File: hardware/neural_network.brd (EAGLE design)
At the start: 31.2 x 39 mm, 32 parts, among them IC1 74AHC1G04DBV, IC2 74AHC1G04DBV, IC3 74AHCT1G14DBV, IC4 74AHCT1G14DBV

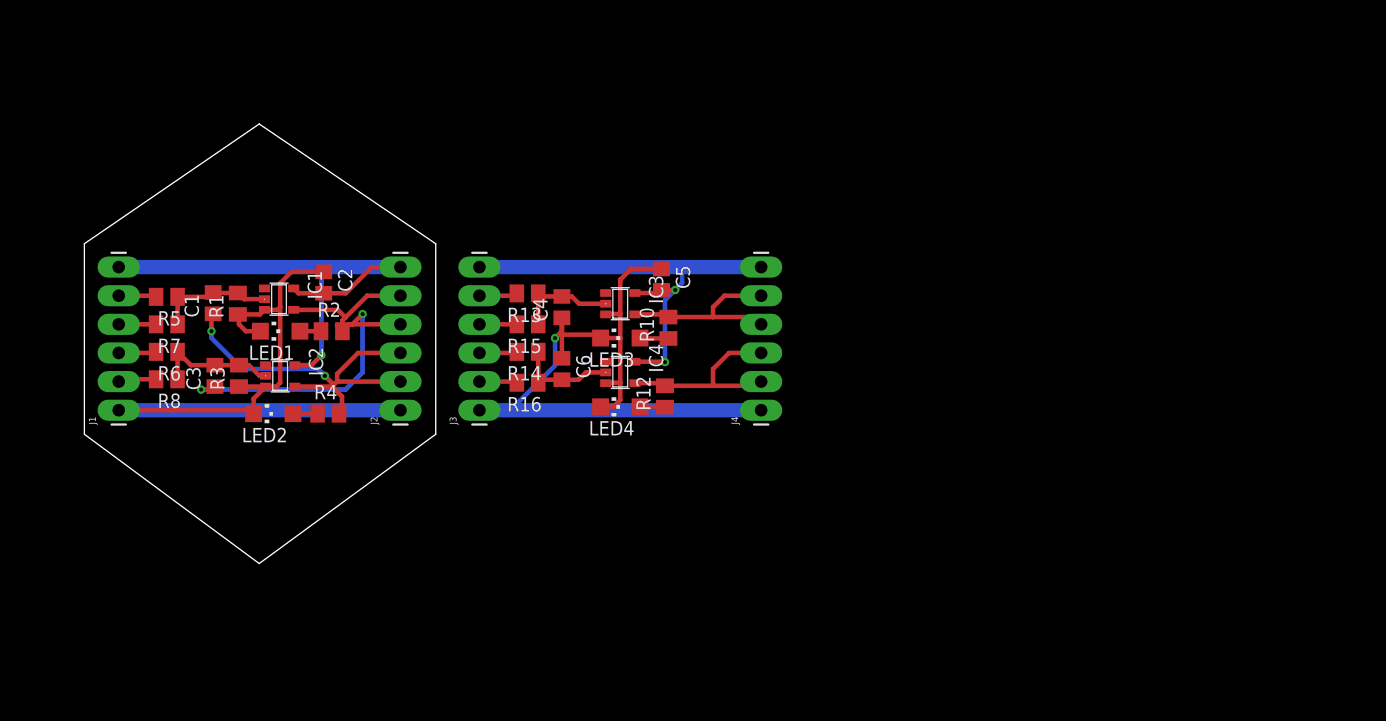
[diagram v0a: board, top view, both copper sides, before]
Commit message: hw
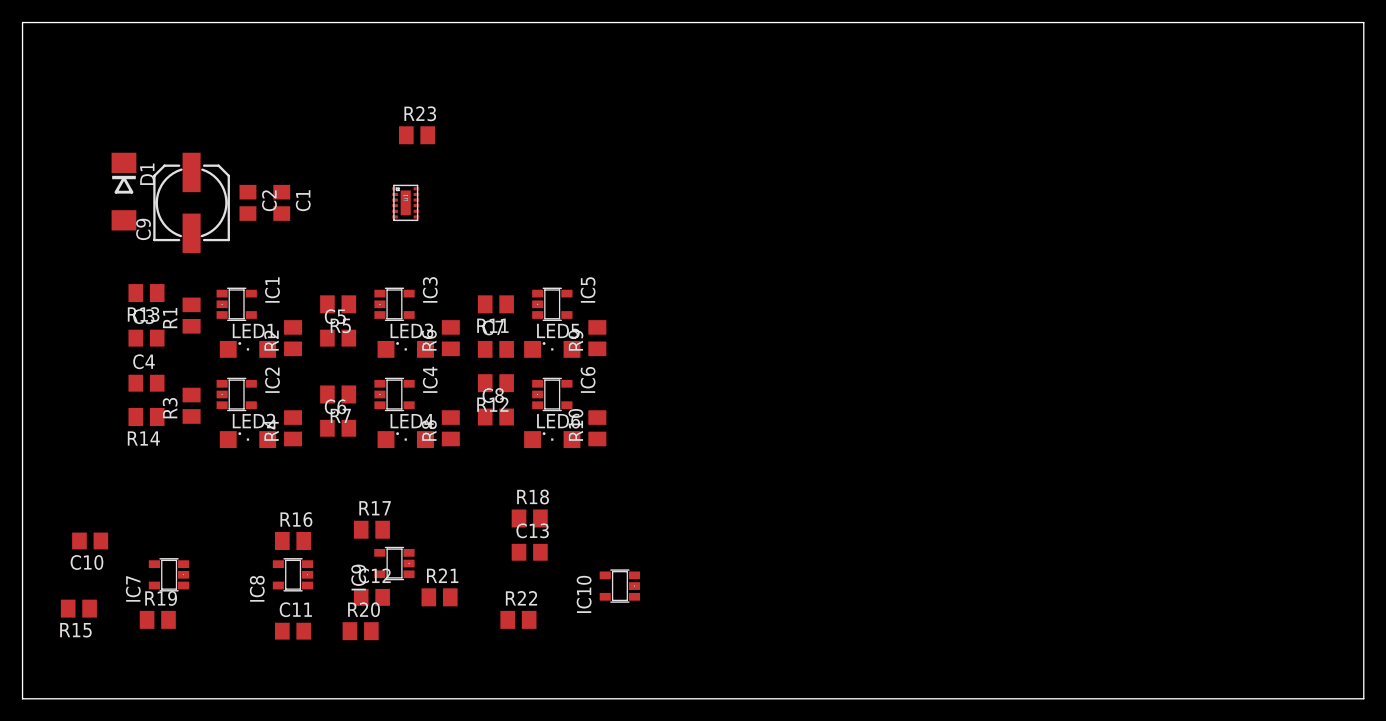
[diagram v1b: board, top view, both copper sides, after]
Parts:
- removed J1, J2, J3, J4: (no value), SparkFun-Connectors:1X06_LONGPADS
- added C10, C11, C12, C13, C7, C8: 100n, resistor:C0805
- added C9: 22uF, resistor:153CLV-0605
- added D1: (no value), diode:DO214AA
- added IC10, IC5, IC6, IC7, IC8, IC9: 74AHC1G14DBV, 74xx-little-de:SOT23-5
- added LED5, LED6: (no value), led:SML1206
- added R11, R17, R18, R19, R20, R21, R22: 1M, resistor:M0805
- added R23, R9: 4k7, resistor:M0805
- added U1: DRV8836, balto:12WSON
- C2: value 100n -> 10uF
- IC1, IC2: value 74AHC1G04DBV -> 74AHC1G14DBV
- IC3, IC4: value 74AHCT1G14DBV -> 74AHC1G14DBV
- LED1, LED2, LED3, LED4: device led:CHIPLED_1206 -> led:SML1206
- R12: value 4k7 -> 1M
- R6, R8: value 1M -> 4k7
- moved R15 47.1 mm to (5.00, 8.00)
- moved C4 37.5 mm to (11.0, 28.0), turned to 0 degrees
- moved R14 34.3 mm to (11.0, 25.0)
- moved R13 33.8 mm to (11.0, 36.0)
- moved C5 29.2 mm to (28.0, 32.0), turned to 0 degrees
- moved R8 25.6 mm to (38.0, 24.0), turned to 90 degrees
- moved R6 25.2 mm to (38.0, 32.0), turned to 90 degrees
- moved R16 25.1 mm to (24.0, 14.0), turned to 0 degrees
- moved C6 20.5 mm to (28.0, 24.0), turned to 0 degrees
- moved IC4 20.1 mm to (33.0, 27.0)
- moved IC3 20.0 mm to (33.0, 35.0)
- moved LED4 19.3 mm to (34.0, 23.0), turned to 0 degrees
- moved LED3 19.1 mm to (34.0, 31.0), turned to 0 degrees
- moved R7 16.4 mm to (28.0, 27.0)
- moved R5 15.2 mm to (28.0, 35.0)
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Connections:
- removed net +3V3: C2.2, C5.2, IC1.5, IC2.5, IC3.5, IC4.5, J1.6, J2.6, J3.6, J4.6
- removed net IN0: J1.5, R5.2
- removed net IN0_: J3.5, R13.2
- removed net IN1: J1.4, R7.2
- removed net IN1_: J3.4, R15.2
- removed net IN2: J1.3, R6.2
- removed net IN2_: J3.3, R14.2
- removed net IN3: J1.2, R8.2
- removed net IN3_: J3.2, R16.2
- removed net N$7 (its old number): LED4.A, R12.1
- removed net OUT0: C3.1, IC1.4, J2.4, J2.5, R2.2
- removed net OUT0_: IC3.4, J4.4, J4.5, R10.2
- removed net OUT1: C1.1, IC2.4, J2.2, J2.3, R4.2
- removed net OUT1_: IC4.4, J4.2, J4.3, R12.2
- new net B_OUT_0: C4.1, IC1.4, R2.2, R5.2, U1.10
- new net B_OUT_1: C3.1, IC2.4, R4.2, R7.2, U1.9
- new net IN_0: R13.2
- new net IN_1: R14.2
- new net N$10: C7.2, IC5.2, R11.1
- new net N$11: LED5.A, R9.1
- new net N$12: C8.2, IC6.2, R12.1
- new net N$13: LED6.A, R10.1
- new net N$14: C10.2, IC7.2, R15.2, R19.1
- new net N$15: C10.1
- new net N$16: IC7.4
- new net N$17: C11.2, IC8.2, R16.2, R20.1
- new net N$18: C11.1
- new net N$19: IC8.4
- new net N$20: C12.2, IC9.2, R17.2, R21.1
- new net N$21: C12.1
- new net N$22: IC9.4
- new net N$23: C13.2, IC10.2, R18.2, R22.1
- new net N$24: C13.1
- new net N$25: IC10.4
- new net N$26: R19.2
- new net N$27: R20.2
- new net N$28: R21.2
- new net N$29: R22.2
- new net N$32: R23.2, U1.12
- new net N$33: U1.3
- new net N$36: U1.2
- new net N$37: U1.4
- new net N$38: U1.5
- new net N$8: C6.2, IC4.2, R7.1
- new net N$9: LED4.A, R8.1
- new net S0_OUT_0: IC3.4, R11.2, R6.2, U1.8
- new net S0_OUT_1: IC4.4, R12.2, R8.2, U1.7
- new net S1_OUT_0: IC5.4, R9.2
- new net S1_OUT_1: IC6.4, R10.2
- new net VCC: D1.A, IC10.5, IC7.5, IC8.5, IC9.5, U1.1
- net GND: now also C1.2, C2.2, C7.1, C8.1, C9.-, IC10.3, IC5.3, IC6.3, IC7.3, IC8.3, IC9.3, LED5.C, LED6.C, R15.1, R16.1, R17.1, R18.1, U1.11, U1.TH; no longer C2.1, C4.1, J1.1, J2.1, J3.1, J4.1
- net N$1: now also C1.1, C2.1, C9.+, D1.C, IC1.5, IC2.5, IC3.5, IC4.5, IC5.5, IC6.5; no longer C1.2, IC1.2, R1.2, R5.1, R7.1
- net N$2: now also C3.2, IC1.2, R1.2; no longer C4.2, IC3.2, R15.1
- net N$3: now also C5.2, IC3.2, R5.1; no longer LED3.A, R10.1
- net N$4: now also C4.2, R14.1; no longer C3.2, R6.1, R8.1
- net N$6: now also LED3.A, R6.1; no longer C6.2, IC4.2, R14.1, R16.1
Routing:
- net GND: track 129.8 -> 0.00 mm, vias 1 -> 0
- net +3V3: track 86.6 -> 0.00 mm, vias 3 -> 0
- net OUT0: track 40.7 -> 0.00 mm, vias 2 -> 0
- net OUT1: track 34.4 -> 0.00 mm, vias 2 -> 0
- net OUT1_: track 17.8 -> 0.00 mm
- net OUT0_: track 17.1 -> 0.00 mm
- net N$4: track 11.1 -> 0.00 mm
- net N$1: track 10.6 -> 0.00 mm
- net N$6: track 9.11 -> 0.00 mm
- net N$2: track 9.11 -> 0.00 mm
- net IN0_: track 3.40 -> 0.00 mm
- net IN3: track 3.40 -> 0.00 mm
- net IN2: track 3.36 -> 0.00 mm
- net IN3_: track 3.36 -> 0.00 mm
- net IN2_: track 3.36 -> 0.00 mm
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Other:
- board size 31.2 x 39 mm -> 119 x 60 mm
